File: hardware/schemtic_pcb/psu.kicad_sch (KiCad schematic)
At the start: 29 parts, among them J1 XT60 Connector, J5 Conn_01x06, Q1 IRF520N, Q2 2N7002, U2 LM2576HVS-ADJ

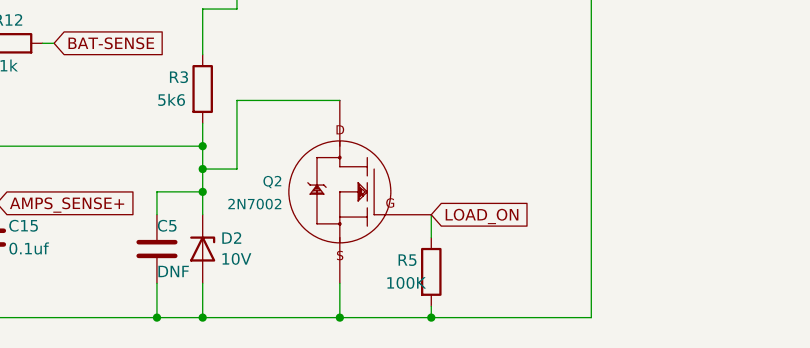
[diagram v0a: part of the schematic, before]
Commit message: Add latest schematic and PCB.
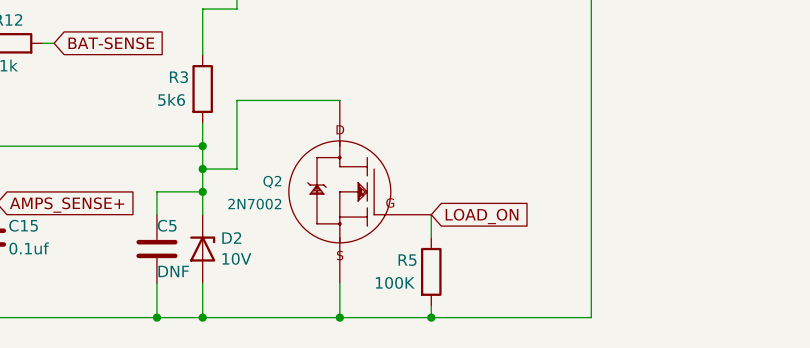
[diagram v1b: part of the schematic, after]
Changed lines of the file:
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@@
       (effects (font (size 1.27 1.27)) (justify left))
     )
-    (property "Value" "100K" (id 1) (at 146.05 157.48 0)
+    (property "Value" "100K" (id 1) (at 144.78 157.48 0)
       (effects (font (size 1.27 1.27)) (justify left))
     )
